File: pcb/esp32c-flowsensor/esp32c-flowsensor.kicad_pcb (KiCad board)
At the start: 2 copper layers, 85.1 x 40 mm, 30 parts, among them J1 NTC1, J2 NTC2, J3 Heater, J4 ALARM, J5 12V In, Q1 BC817, Q2 IRF540N, Q3 BC817, U1 AMS1117-5.0, U2 esp32-c3-ebay

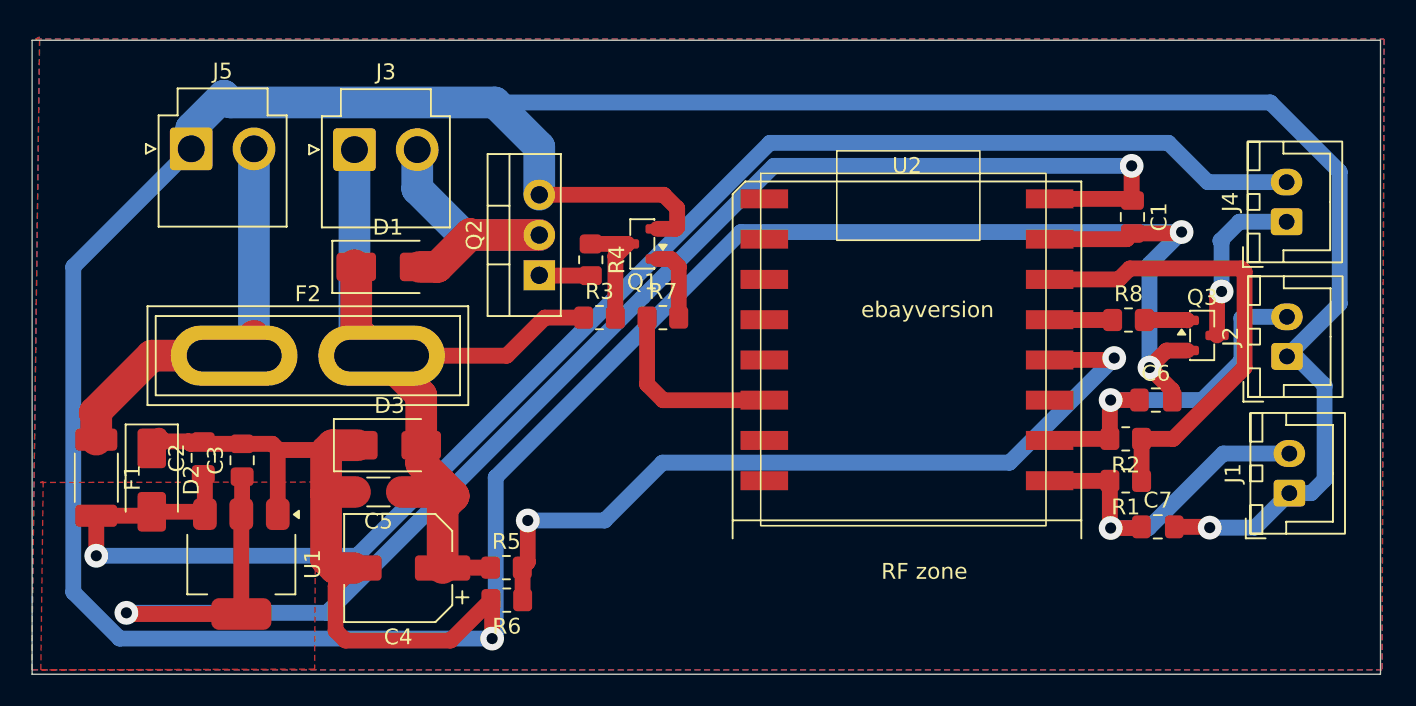
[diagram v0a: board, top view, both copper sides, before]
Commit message: Pcb update
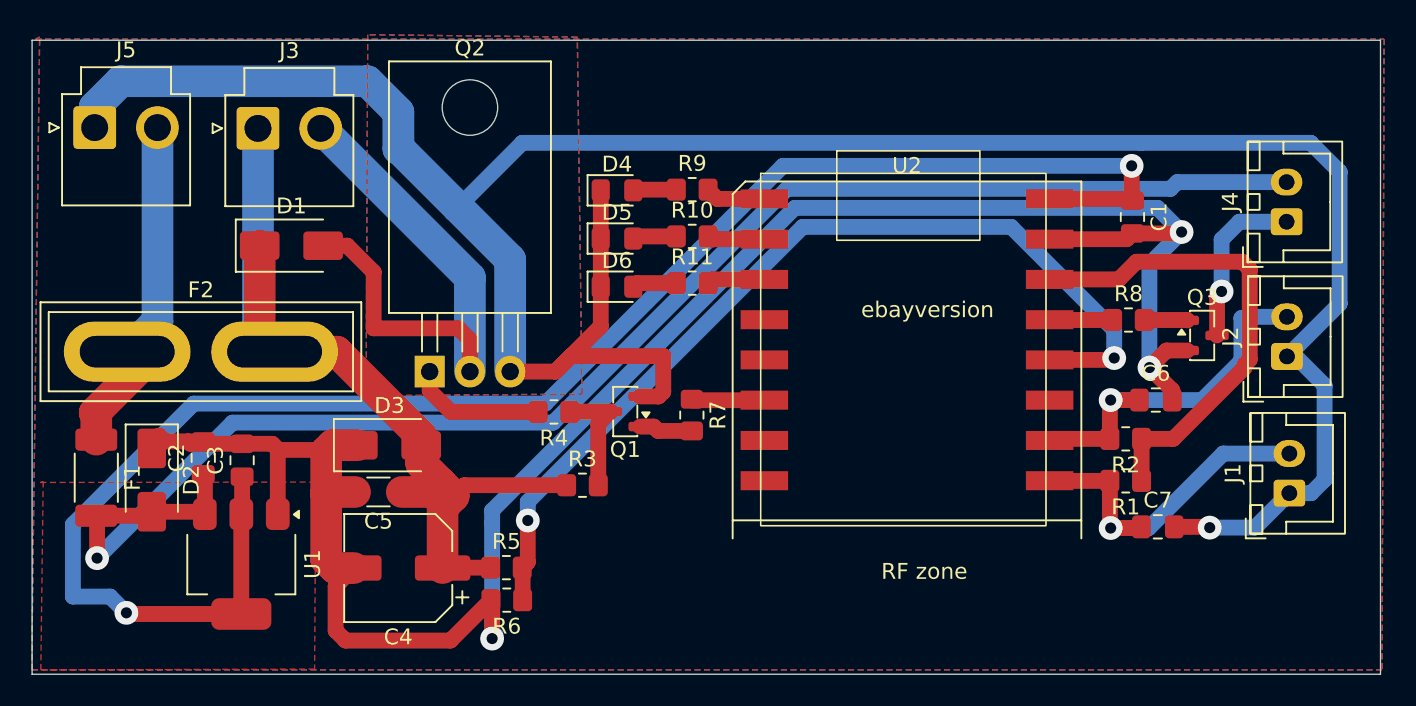
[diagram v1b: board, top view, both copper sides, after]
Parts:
- added D4: LED, LED_SMD:LED_0805_2012Metric_Pad1.15x1.40mm_HandSolder, F.Cu at (98.5, 69.8)
- added D5: LED, LED_SMD:LED_0805_2012Metric_Pad1.15x1.40mm_HandSolder, F.Cu at (98.5, 72.9)
- added D6: LED, LED_SMD:LED_0805_2012Metric_Pad1.15x1.40mm_HandSolder, F.Cu at (98.5, 75.9)
- added R10: 10K, Resistor_SMD:R_0805_2012Metric_Pad1.20x1.40mm_HandSolder, F.Cu at (103.2, 72.7)
- added R11: 10K, Resistor_SMD:R_0805_2012Metric_Pad1.20x1.40mm_HandSolder, F.Cu at (103.2, 75.7)
- added R9: 10K, Resistor_SMD:R_0805_2012Metric_Pad1.20x1.40mm_HandSolder, F.Cu at (103.2, 69.8)
- Q2: footprint Package_TO_SOT_THT:TO-220-3_Vertical -> Package_TO_SOT_THT:TO-220-3_Horizontal_TabDown
- moved R3 10.6 mm to (96.3, 88.4)
- moved Q1 10.6 mm to (99.0, 83.8)
- moved R4 9.88 mm to (94.5, 83.8), turned to 180 degrees
- moved Q2 9.20 mm to (86.7, 81.3), turned to 0 degrees
- moved F2 6.75 mm to (67.6, 80.0)
- moved R7 6.42 mm to (103.2, 84.0), turned to -90 degrees
- moved D1 6.24 mm to (78.0, 73.3)
- moved J3 6.24 mm to (75.8, 65.9)
- moved J5 6.24 mm to (65.5, 65.9)
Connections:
- U2 pad 1: unconnected-(U2-gpio5-Pad1) -> STILL_LED
- U2 pad 2: unconnected-(U2-gop6-Pad2) -> AIR_LED
- U2 pad 3: unconnected-(U2-gpio7-Pad3) -> FLOW_LED
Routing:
- net GND: track 317.8 -> 290.2 mm
- net HEATER_POWER: track 19.8 -> 35.1 mm
- net 5V: track 98.5 -> 107.8 mm
- net 12V_SENSE: track 50.6 -> 59.1 mm
- net HEATER_PWM: track 12.0 -> 4.60 mm
- net 12IN: track 27.4 -> 21.8 mm
- net Net-(Q2-G): track 3.26 -> 8.60 mm
- net STILL_LED: track 0.00 -> 3.79 mm
- net FLOW_LED: track 0.00 -> 3.65 mm
- net AIR_LED: track 0.00 -> 3.62 mm
- net Net-(D6-A): track 0.00 -> 2.81 mm
- net Net-(D5-A): track 0.00 -> 2.78 mm
- net Net-(D4-A): track 0.00 -> 2.74 mm
- net 12VF: track 99.0 -> 96.6 mm
- net Net-(Q1-B): track 4.77 -> 3.38 mm
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- added copper zone on B.Cu, net HEATER_POWER
- added copper zone on F.Cu, net HEATER_POWER
